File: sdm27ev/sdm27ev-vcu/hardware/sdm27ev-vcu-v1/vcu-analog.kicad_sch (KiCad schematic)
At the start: 90 parts, among them IC15 TPD4E05U06QDQARQ1, IC16 TPD4E05U06QDQARQ1, Q2 TPS2058AD, Q3 TPS2058AD, U4 TCA6408ARSV, U5 TLV9064IRUCR, U6 TLV9064IRUCR, U7 TCA6408ARSV

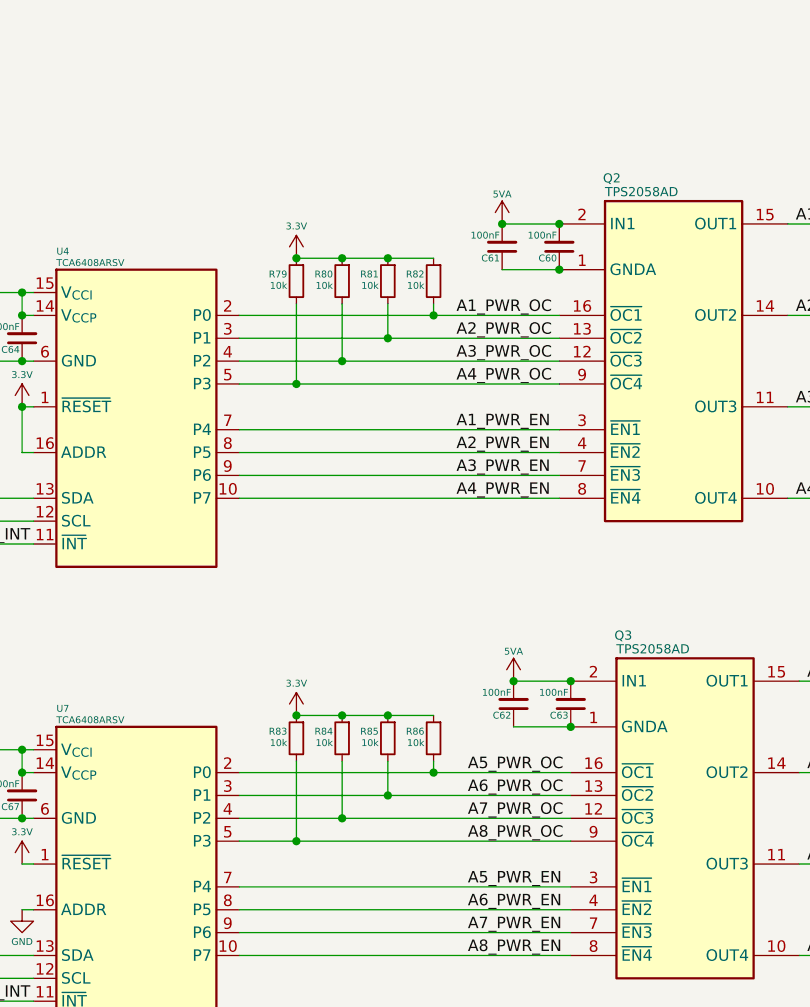
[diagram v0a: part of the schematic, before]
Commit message: Minor QOL VCU edits before design review
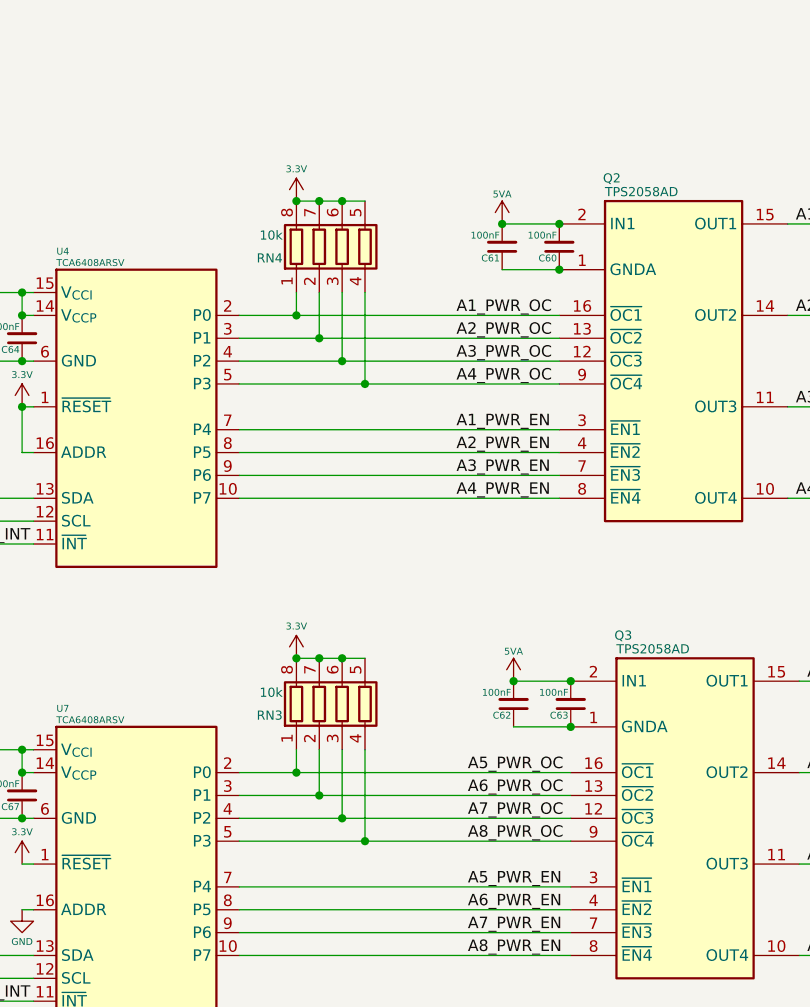
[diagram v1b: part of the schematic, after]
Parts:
- removed R79, R80, R81, R82, R83, R84, R85, R86: 10k, Resistor_SMD:R_0603_1608Metric, symbol Device:R_Small
- added RN3, RN4: 10k, Resistor_SMD:R_Array_Convex_4x0603, symbol Device:R_Pack04
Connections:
- net 3.3V: now also RN3.5 (R4.2), RN3.6 (R3.2), RN3.7 (R2.2), RN3.8 (R1.2), RN4.5 (R4.2), RN4.6 (R3.2), RN4.7 (R2.2), RN4.8 (R1.2)
- net A1_PWR_OC: now also RN4.1 (R1.1)
- net A2_PWR_OC: now also RN4.2 (R2.1)
- net A3_PWR_OC: now also RN4.3 (R3.1)
- net A4_PWR_OC: now also RN4.4 (R4.1)
- net A5_PWR_OC: now also RN3.1 (R1.1)
- net A6_PWR_OC: now also RN3.2 (R2.1)
- net A7_PWR_OC: now also RN3.3 (R3.1)
- net A8_PWR_OC: now also RN3.4 (R4.1)
